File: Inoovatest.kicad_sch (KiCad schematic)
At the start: 13 parts, among them J1 USB_C Charging port

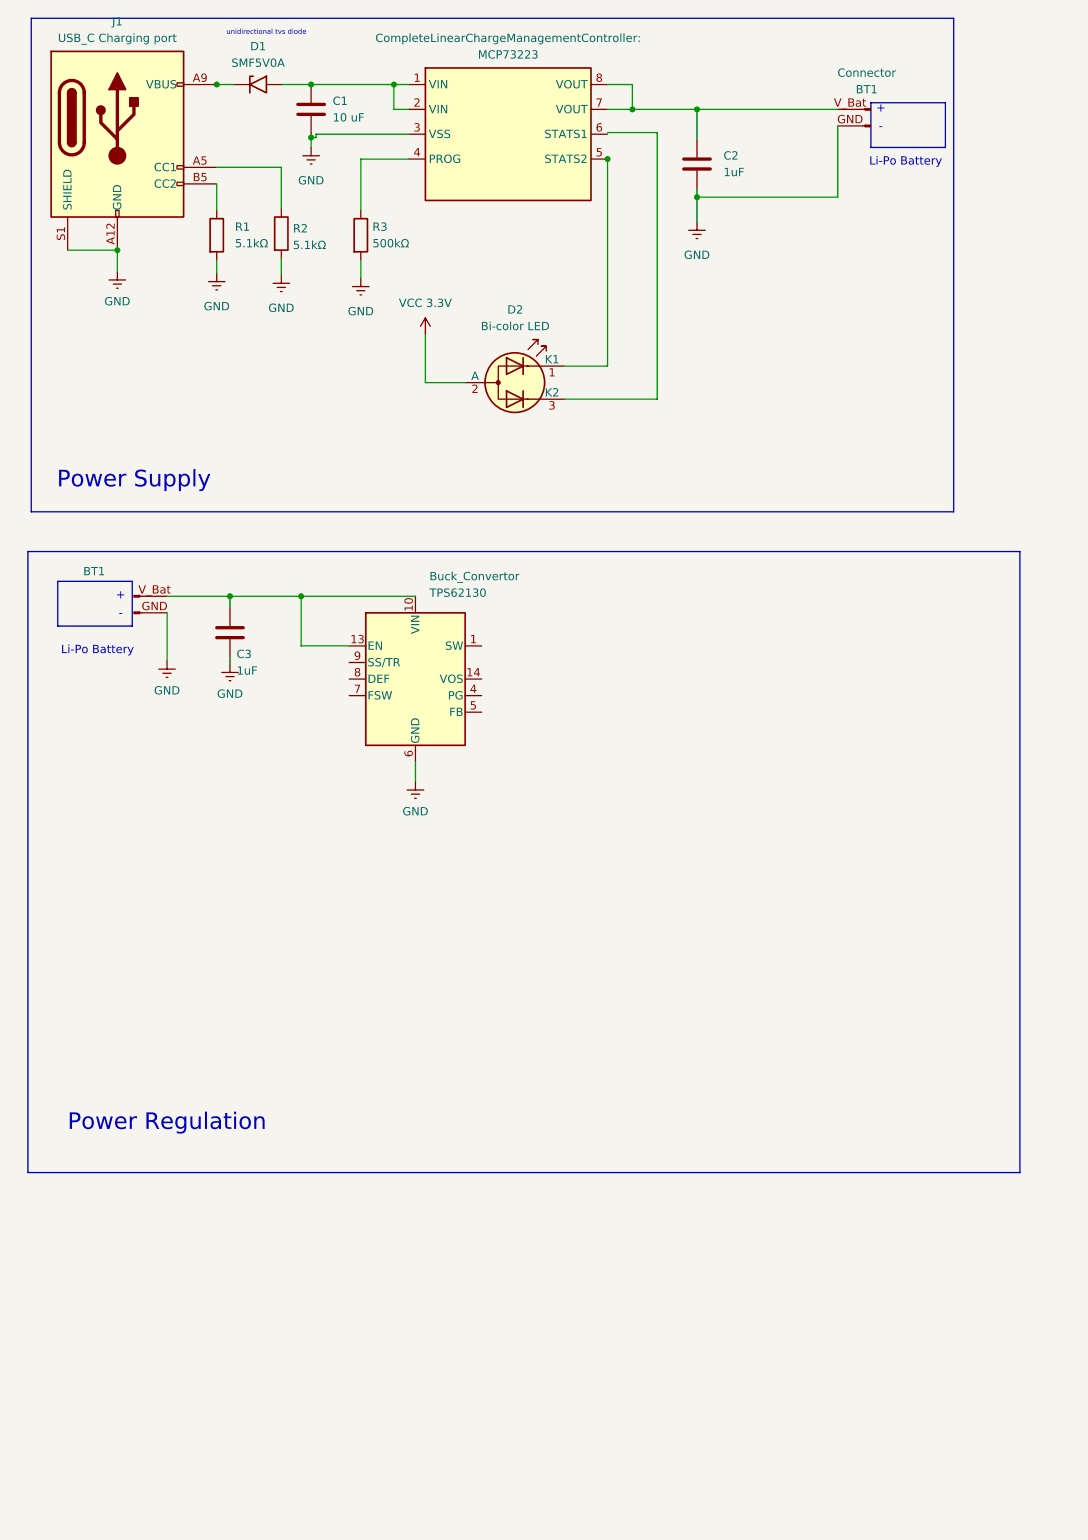
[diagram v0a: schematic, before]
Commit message: Add files via upload
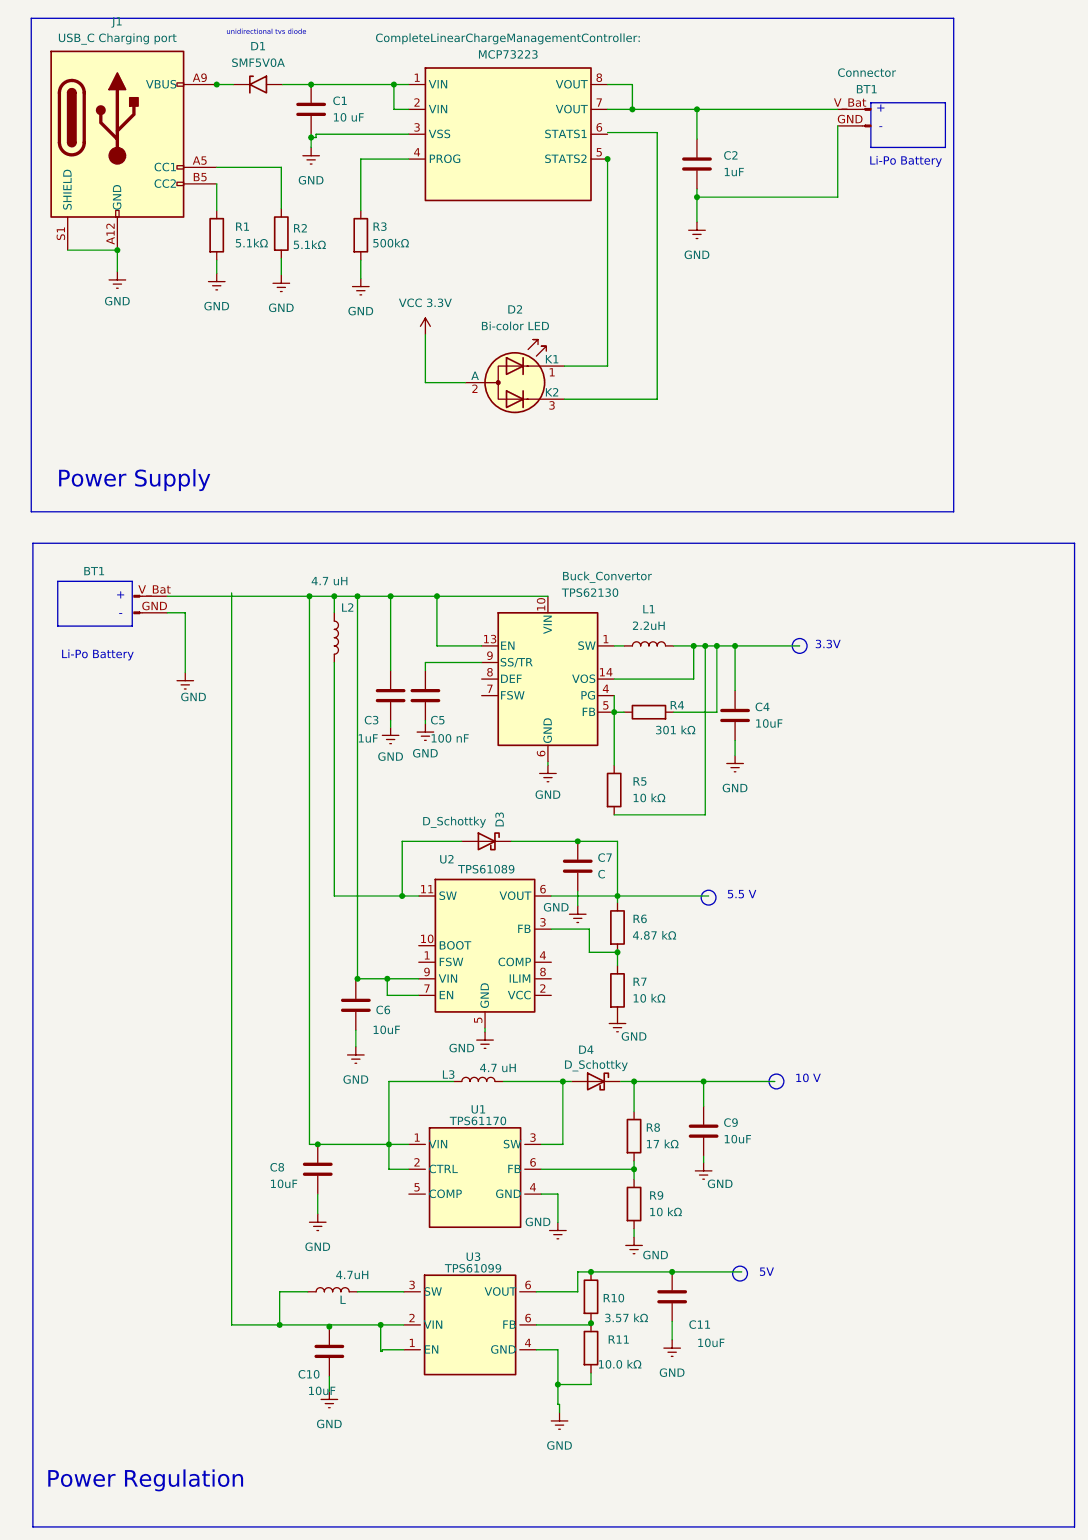
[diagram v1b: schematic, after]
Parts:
- added 4.7uH: L, symbol Device:L
- added C10, C11, C4, C6, C8, C9: 10uF, symbol Device:C
- added C5: 100 nF, symbol Device:C
- added C7: C, symbol Device:C
- added D3, D4: D_Schottky, symbol Device:D_Schottky
- added L1: 2.2uH, symbol Device:L
- added L2, L3: 4.7 uH, symbol Device:L
- added R10: 3.57 kΩ, symbol Device:R
- added R11: 10.0 kΩ, symbol Device:R
- added R4: 301 kΩ, symbol Device:R
- added R5, R7, R9: 10 kΩ, symbol Device:R
- added R6: 4.87 kΩ, symbol Device:R
- added R8: 17 kΩ, symbol Device:R
- added U1: TPS61170, Package_TO_SOT_SMD:SOT-23-6, symbol Driver_LED:TPS61165DBV
- added U2: TPS61089, Package_DFN_QFN:Texas_VQFN-RNR0011A-11, symbol Regulator_Switching:TPS61089
- added U3: TPS61099, Package_TO_SOT_SMD:SOT-23-6, symbol Driver_LED:TPS61165DBV
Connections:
- net GND: now also C10.2, C11.2, C4.2, C5.2, C6.2, C7.2, C8.2, C9.2, R11.2, R7.2, R9.2, U1.4 (GND), U2.5 (GND), U3.4 (GND)
- net at Buck_Convertor.10 (VIN), Buck_Convertor.11 (VIN), Buck_Convertor.12 (VIN)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: now also C6.1, C8.1, L2.1, L3.2, U1.1 (VIN), U1.2 (CTRL), U2.7 (EN), U2.9 (VIN)
- net at Buck_Convertor.1 (SW), Buck_Convertor.2 (SW), Buck_Convertor.3 (SW): now also L1.1
- net at Buck_Convertor.14 (VOS): now also C4.1, L1.2, R4.2, R5.2
- net at Buck_Convertor.4 (PG): now also Buck_Convertor.5 (FB), R4.1, R5.1
- net at Buck_Convertor.9 (SS/TR): now also C5.1
- new net: 4.7uH.1, C10.1, U3.1 (EN), U3.2 (VIN)
- new net: 4.7uH.2, U3.3 (SW)
- new net: C11.1, R10.1, U3.6 (FB)
- new net: R10.2, R11.1, U3.6 (FB)
- new net: C9.1, D4.1 (K), R8.1
- new net: D4.2 (A), L3.1, U1.3 (SW)
- new net: D3.2 (A), L2.2, U2.11 (SW)
- new net: R6.2, R7.1, U2.3 (FB)
- new net: C7.1, D3.1 (K), R6.1, U2.6 (VOUT)
- new net: R8.2, R9.1, U1.6 (FB)
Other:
- note added: "10 V"
- note added: "3.3V"
- note added: "5.5 V"
- note added: "5V"
- moved on the sheet: Buck_Convertor, C3
